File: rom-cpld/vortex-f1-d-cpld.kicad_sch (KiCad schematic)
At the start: 28 parts, among them J1 JTAG, J2 Floppy, SW1 SW_DIP_x04, U1 37C65, U2 XC9572XL, U3 AZ1117-3.3, U5 AM29F010, Y1 16MHz

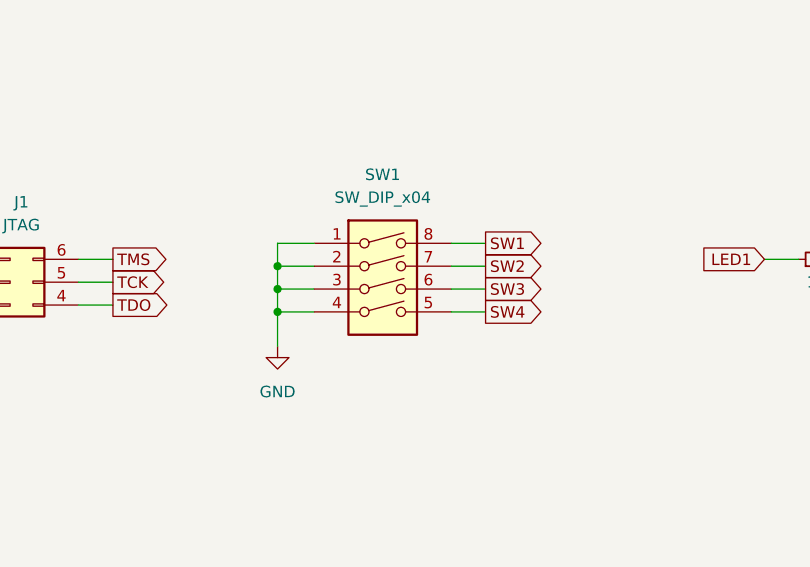
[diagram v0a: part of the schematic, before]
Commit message: v1.0 sent to jlcpcb for production
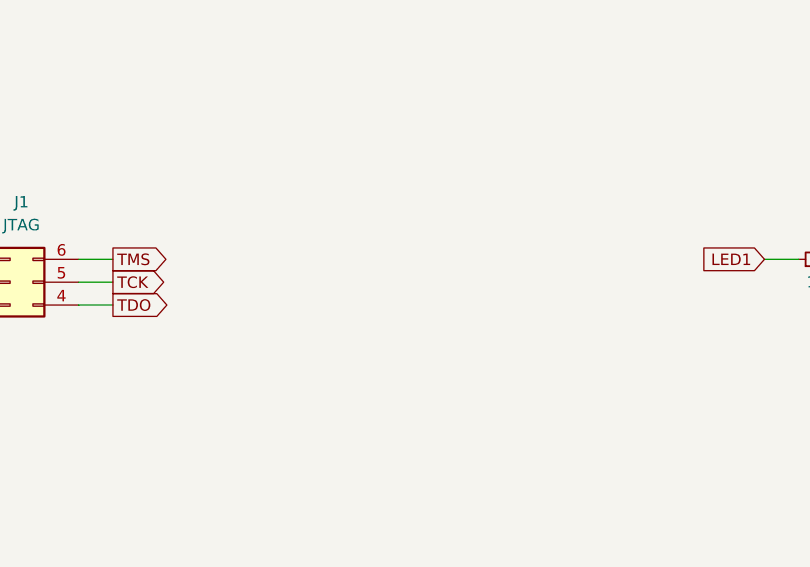
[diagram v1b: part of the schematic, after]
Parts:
- removed SW1: SW_DIP_x04, Button_Switch_THT:SW_DIP_SPSTx04_Slide_6.7x11.72mm_W7.62mm_P2.54mm_LowProfile, symbol Switch:SW_DIP_x04
- Y1: footprint Crystal:Crystal_HC49-U_Horizontal -> Crystal:Crystal_SMD_7050-4Pin_7.0x5.0mm

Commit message: add new vhdl code
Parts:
- removed J1: JTAG, Connector_PinHeader_2.54mm:PinHeader_2x03_P2.54mm_Vertical, symbol Connector_Generic:Conn_02x03_Counter_Clockwise
- added J3: Micro_SD_Card, project:J_SD_Card-micro_socket_A, symbol Connector:Micro_SD_Card
- added U4: Pico, MCU_RaspberryPi_and_Boards:RPi_Pico_SMD_TH, symbol MCU_RaspberryPi_and_Boards:Pico
- R2, R3, R4, R5, R6: value 1k -> 150
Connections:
- net FLTR/STEP is gone; now on net ~{INT}: U2.2 (I/O/GTS2)
- net FLT/TRK0 is gone; now on net ~{WR}: U2.4 (P4)
- net SW1 is gone; now on net D3: U2.12 (P12)
- net SW2 is gone; now on net D4: U2.13 (P13)
- net SW3 is gone; now on net D6: U2.16 (I/O/GCK2)
- net US0 is gone; now on net ~{RD}: U2.6 (P6)
- net US1 is gone; now on net ~{IORQ}: U2.5 (I/O/GTS1)
- net WE is gone; now on net ~{M1}: U2.7 (P7)
- net ~{DS0'} is gone; now on net A8: U2.31 (P31)
- net ~{DS1'} is gone; now on net A7: U2.27 (P27)
- net ~{DS2'} is gone; now on net A6: U2.25 (P25)
- net ~{DS3'} is gone; now on net A9: U2.32 (P32)
- net ~{RW}/SEEK is gone; now on net ~{ROMEN}: U2.1 (P1)
- net +3.3V: now also J3.4 (VDD)
- net A0: now also U2.18 (P18); no longer U2.45 (P45)
- net A1: now also U2.19 (P19); no longer U2.44 (P44)
- net A10: now also U2.33 (P33); no longer U2.35 (P35)
- net A11: now also U2.34 (P34)
- net A12: now also U2.35 (P35)
- net A13: now also U2.36 (P36); no longer U2.34 (P34)
- net A14: now also U2.38 (P38)
- net A15: now also U2.39 (P39); no longer U2.33 (P33)
- net A2: now also U2.20 (P20); no longer U2.43 (P43)
- net A3: now also U2.22 (P22); no longer U2.42 (P42)
- net A4: now also U2.23 (P23); no longer U2.40 (P40)
- net A5: now also U2.24 (P24); no longer U2.39 (P39)
- net A6: no longer U2.38 (P38)
- net A7: no longer U2.36 (P36)
- net A8: no longer U2.18 (P18)
- net A9: no longer U2.17 (I/O/GCK3)
- net CLK4: no longer U2.58 (P58)
- net D0: now also U2.9 (P9), U4.21 (GPIO16); no longer U2.46 (P46)
- net D1: now also U2.10 (P10), U4.22 (GPIO17)
- net D2: now also U2.11 (P11), U4.24 (GPIO18)
- net D3: now also U4.25 (GPIO19)
- net D4: now also U4.26 (GPIO20)
- net D5: now also U2.15 (I/O/GCK1), U4.27 (GPIO21)
- net D6: now also U4.29 (GPIO22)
- net D7: now also U2.17 (I/O/GCK3), U4.31 (GPIO26_ADC0)
- net GND: now also J3.6 (VSS)
- net LED1: no longer U2.15 (I/O/GCK1)
- net MTRON: no longer U2.24 (P24)
- net READY: no longer U2.51 (P51)
- net RESET: no longer U2.8 (P8)
- net ROMA14: now also U2.64 (I/O/GSR); no longer U2.59 (P59)
- net ROMA15: now also U2.59 (P59); no longer U2.64 (I/O/GSR)
- net ROMA16: now also U2.60 (P60); no longer U2.63 (P63)
- net STEP: no longer U2.20 (P20)
- net SW4: no longer U2.19 (P19)
- net TCK: now also U4.2 (GPIO1)
- net TDI: now also U4.5 (GPIO3)
- net TDO: now also U4.4 (GPIO2)
- net TMS: now also U4.1 (GPIO0)
- net TRK00: no longer U2.23 (P23)
- net WGATE: no longer U2.22 (P22)
- net ~{FDCCS}: no longer U2.11 (P11)
- net ~{IORD}: no longer U2.9 (P9)
- net ~{IORQ}: no longer U2.48 (P48)
- net ~{IOWR}: no longer U2.10 (P10)
- net ~{MREQ}: now also U2.8 (P8); no longer U2.47 (P47)
- net ~{RD}: no longer U2.49 (P49)
- net ~{ROMEN}: no longer U2.52 (P52)
- net ~{ROMOE}: now also U2.63 (P63); no longer U2.61 (P61)
- net ~{ROMWE}: now also U2.61 (P61); no longer U2.60 (P60)
- net ~{RSET}: now also U2.52 (P52); no longer U2.56 (P56)
- net ~{WR}: no longer U2.50 (P50)
- net ~{CCR_WR} renamed ~{LDCR}
- net ~{DOR_WR} renamed ~{LDOR}
- new net PICO10: U2.45 (P45), U4.14 (GPIO10)
- new net PICO11: U2.46 (P46), U4.15 (GPIO11)
- new net PICO12: U2.44 (P44), U4.16 (GPIO12)
- new net PICO13: U2.43 (P43), U4.17 (GPIO13)
- new net PICO14: U2.42 (P42), U4.19 (GPIO14)
- new net PICO15: U2.40 (P40), U4.20 (GPIO15)
- new net SDCK: J3.5 (CLK), U4.9 (GPIO6)
- new net SDCS: J3.2 (DAT3/CD), U4.12 (GPIO9)
- new net SDDETECT: J3.9 (DETECT), U4.7 (GPIO5)
- new net SDMISO: J3.7 (DAT0), U4.11 (GPIO8)
- new net SDMOSI: J3.3 (CMD), U4.10 (GPIO7)
- no-connect marks 6 -> 23
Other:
- moved on the sheet: C13, C14, D1, J2, S1, U1, U2, U5, Y1
